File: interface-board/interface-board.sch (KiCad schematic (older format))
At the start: 25 parts, among them J1 HECS, J10 AUX, J11 UART, J12 NTC1, J13 NTC1, J14 RJ45, J2 CASEFAN1, J3 CASEFAN2, J4 AMPSEAL_PWR, J5 AMPSEAL_MAIN, J6 HV+, J7 HV-, J8 IMD, J9 TSMP

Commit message: Updated main connector and pinout
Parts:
- removed J4: AMPSEAL_PWR, Connector_JST:JST_ZE_B08B-ZESK-1D_1x08_P1.50mm_Vertical, symbol Connector_Generic:Conn_01x08
- removed J5: AMPSEAL_MAIN, CustomFootprints:AMPSEAL 776266-1 14-PIN, symbol Connector_Generic:Conn_01x14
- removed JP1: Jumper, Jumper:SolderJumper-2_P1.3mm_Open_RoundedPad1.0x1.5mm, symbol Jumper:SolderJumper_2_Open
- added J16: Conn_01x23, 1-776087-1:TE_1-776087-1, symbol Connector_Generic:Conn_01x23
- J10: symbol Connector_Generic:Conn_01x04 -> Connector_Generic:Conn_01x03
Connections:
- net +12V: now also J16.14 (Pin_14), J16.6 (Pin_6)
- net +5V: now also J16.23 (Pin_23)
- net CAN+: now also J16.11 (Pin_11)
- net CAN-: now also J16.12 (Pin_12)
- net FANOUT1: now also J16.8 (Pin_8)
- net FANOUT2: now also J16.15 (Pin_15)
- net FANOUT3: now also J16.7 (Pin_7)
- net GND: now also J16.13 (Pin_13), J16.3 (Pin_3), J16.4 (Pin_4), J16.5 (Pin_5)
- net IMD_AN1: now also J16.20 (Pin_20)
- net IMD_AN2: now also J16.21 (Pin_21)
- net IMD_AN3: now also J16.22 (Pin_22)
- net SHDN_LOOP_OUT: now also J16.1 (Pin_1), J16.10 (Pin_10), J16.16 (Pin_16), J16.2 (Pin_2), J16.9 (Pin_9)
- net at J10.3 (Pin_3), JP2.1 (A): now also J16.17 (Pin_17)
- net at J10.2 (Pin_2), JP3.1 (A): now also J16.18 (Pin_18)
- net at J10.1 (Pin_1), JP4.1 (A): now also J16.19 (Pin_19)
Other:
- note removed: "Shutdown loop in = 12V bus"
- moved on the sheet: C1, C2, JP2, JP3, JP4

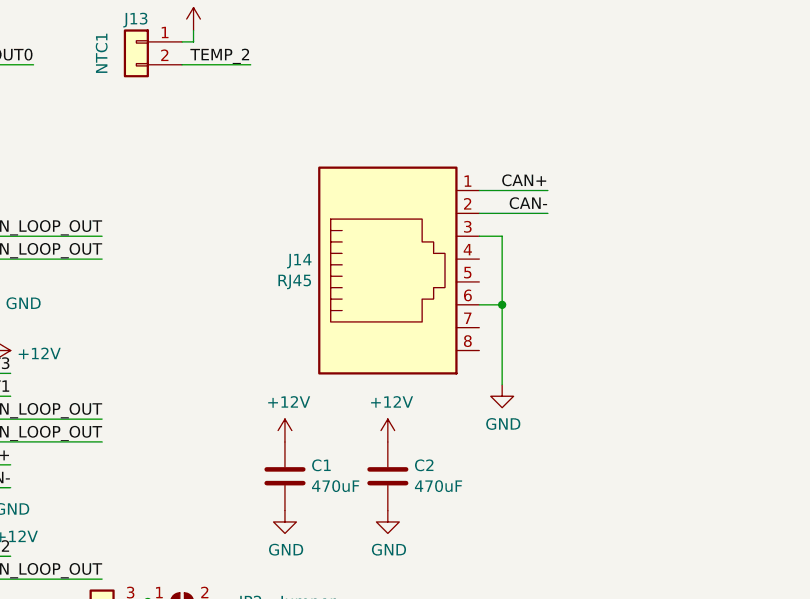
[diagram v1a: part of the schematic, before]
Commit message: Added IMD LV connector
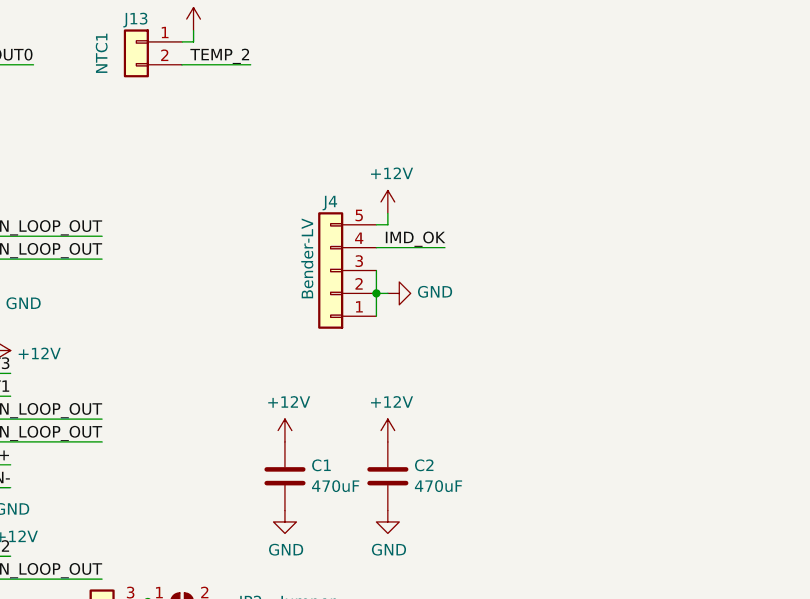
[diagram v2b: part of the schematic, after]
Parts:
- removed J14: RJ45, Connector_RJ:RJ45_Amphenol_54602-x08_Horizontal, symbol Connector:RJ45
- added J4: Bender-LV, Connector_Molex:Molex_KK-254_AE-6410-05A_1x05_P2.54mm_Vertical, symbol Connector_Generic:Conn_01x05
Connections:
- net +12V: now also J4.5 (Pin_5)
- net GND: now also J4.1 (Pin_1), J4.2 (Pin_2), J4.3 (Pin_3)
- new net IMD_OK: J4.4 (Pin_4)
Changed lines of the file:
@@
 Text Label 2450 3300 2    50   ~ 0
 UART_TX
-$Comp
-L Connector:RJ45 J14
-U 1 1 5C565B8C
-P 3000 5550
-F 0 "J14" H 2670 5554 50  0000 R CNN
-F 1 "RJ45" H 2670 5645 50  0000 R CNN
-F 2 "Connector_RJ:RJ45_Amphenol_54602-x08_Horizontal" V 3000 5575 50  0001 C CNN
-F 3 "~" V 3000 5575 50  0001 C CNN
-	1    3000 5550
-	1    0    0    1
-$EndComp
-$Comp
-L power:GND #PWR018
-U 1 1 5C569DF7
-P 3500 6100
-F 0 "#PWR018" H 3500 5850 50  0001 C CNN
-F 1 "GND" H 3505 5927 50  0000 C CNN
-F 2 "" H 3500 6100 50  0001 C CNN
-F 3 "" H 3500 6100 50  0001 C CNN
-	1    3500 6100
-	1    0    0    -1
-$EndComp
-Wire Wire Line
-	3500 6100 3500 5750
-Wire Wire Line
-	3500 5750 3500 5450
-Connection ~ 3500 5750
-Wire Wire Line
-	3400 5250 3700 5250
-Wire Wire Line
-	3400 5350 3700 5350
 Wire Wire Line
 	4600 1350 4300 1350
@@
 CAN+
 Text Label 4300 1450 0    50   ~ 0
-CAN-
-Text Label 3700 5250 2    50   ~ 0
-CAN+
-Text Label 3700 5350 2    50   ~ 0
 CAN-
 Connection ~ 1700 1500
@@
 Text Label 2400 4700 2    50   ~ 0
 TEMP_2
-Wire Wire Line
-	3400 5450 3500 5450
-Wire Wire Line
-	3400 5750 3500 5750
 $Comp
 L Device:C C1
@@
 Wire Wire Line
 	1150 6750 1000 6750
+$Comp
+L Connector_Generic:Conn_01x05 J4
+U 1 1 5C4FC040
+P 2750 5600
+F 0 "J4" H 2750 5300 50  0000 C CNN
+F 1 "Bender-LV" V 2850 5550 50  0000 C CNN
+F 2 "Connector_Molex:Molex_KK-254_AE-6410-05A_1x05_P2.54mm_Vertical" H 2750 5600 50  0001 C CNN
+F 3 "~" H 2750 5600 50  0001 C CNN
+	1    2750 5600
+	-1   0    0    1
+$EndComp
+$Comp
+L power:GND #PWR0105
+U 1 1 5C509587
+P 3000 5700
+F 0 "#PWR0105" H 3000 5450 50  0001 C CNN
+F 1 "GND" V 3005 5572 50  0000 R CNN
+F 2 "" H 3000 5700 50  0001 C CNN
+F 3 "" H 3000 5700 50  0001 C CNN
+	1    3000 5700
+	0    -1   -1   0
+$EndComp
+Wire Wire Line
+	2950 5600 2950 5700
+Connection ~ 2950 5700
+Wire Wire Line
+	2950 5700 2950 5800
+Wire Wire Line
+	2950 5700 3000 5700
+Wire Wire Line
+	2950 5500 3250 5500
+Text Label 3250 5500 2    50   ~ 0
+IMD_OK
+$Comp
+L power:+12V #PWR0106
+U 1 1 5C51B056
+P 3000 5350
+F 0 "#PWR0106" H 3000 5200 50  0001 C CNN
+F 1 "+12V" H 3015 5523 50  0000 C CNN
+F 2 "" H 3000 5350 50  0001 C CNN
+F 3 "" H 3000 5350 50  0001 C CNN
+	1    3000 5350
+	1    0    0    -1
+$EndComp
+Wire Wire Line
+	3000 5350 3000 5400
+Wire Wire Line
+	3000 5400 2950 5400
 $EndSCHEMATC
